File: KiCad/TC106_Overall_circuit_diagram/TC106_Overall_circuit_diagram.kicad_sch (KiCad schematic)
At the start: 52 parts, among them J1 JST_VH_01x05, J10 JST_VH_01x05, J1_24V1 JST_VH_01x04, J1_CN1 JST_VH_01x03, J2 JST_VH_01x05, J2_CN1 JST_VH_01x02, J3 JST_VH_01x05, J3_CN1 JST_VH_01x02, J4 JST_VH_01x05, J4_CN2 JST_VH_01x02, J5 JST_VH_01x05, J5_CN2 JST_VH_01x03, J6 JST_VH_01x05, J7 JST_VH_01x05, J8 JST_VH_01x05, J9 Conn_02x02_Odd_Even, Q1 DTC143E, Q2 DTC143E, Q3 2SD1863, Q5 DTC143E, U1 MC34063AP, U2 PIC16F73-ISP, U3 Dummy dsPic33FJ16MC102, U5 DC-DC_Converter

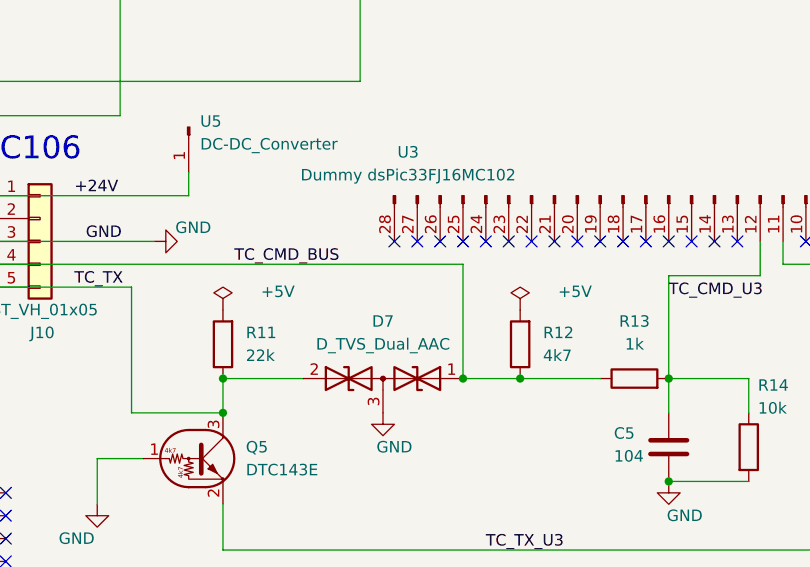
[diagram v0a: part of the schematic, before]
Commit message: UPDATE
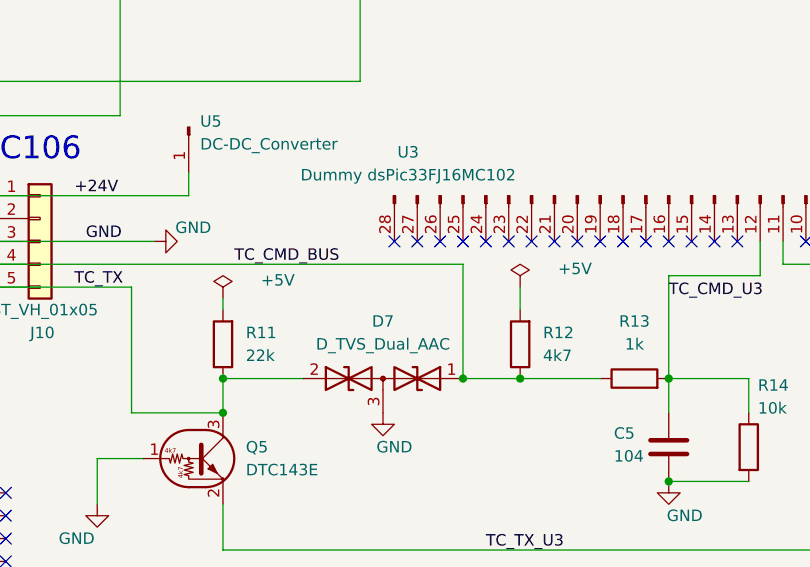
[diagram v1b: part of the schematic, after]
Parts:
- U3: footprint dsPIC33FJ16MC102:SOP65P780X200-28N -> dsPic33FJ16MC102:SOP65P780X200-28N
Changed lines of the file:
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@@
 	(wire
 		(pts
+			(xy 194.31 134.62) (xy 194.31 135.89)
+		)
+		(stroke
+			(width 0)
+			(type default)
+		)
+	)
+	(wire
+		(pts
 			(xy 129.54 142.24) (xy 151.13 142.24)
 		)
@@
 	(wire
 		(pts
+			(xy 227.33 133.35) (xy 227.33 135.89)
+		)
+		(stroke
+			(width 0)
+			(type default)
+		)
+	)
+	(wire
+		(pts
 			(xy 142.24 91.44) (xy 46.99 91.44)
 		)
@@
 	(symbol
 		(lib_id "power:PWR_FLAG")
-		(at 227.33 135.89 0)
+		(at 227.33 133.35 0)
 		(unit 1)
 		(exclude_from_sim no)
@@
 		(dnp no)
 		(property "Reference" "#U11_POWER_5V01"
-			(at 227.33 133.985 0)
+			(at 227.33 131.445 0)
 			(effects
 				(font
@@
 		)
 		(property "Value" "+5V"
-			(at 233.426 133.858 0)
+			(at 233.426 131.318 0)
 			(effects
 				(font
@@
 		)
 		(property "Footprint" ""
-			(at 227.33 135.89 0)
+			(at 227.33 133.35 0)
 			(effects
 				(font
@@
 		)
 		(property "Datasheet" "~"
-			(at 227.33 135.89 0)
+			(at 227.33 133.35 0)
 			(effects
 				(font
@@
 		)
 		(property "Description" "Special symbol for telling ERC where power comes from"
-			(at 227.33 135.89 0)
+			(at 227.33 133.35 0)
 			(effects
 				(font
@@
 			)
 		)
-		(property "Footprint" "dsPIC33FJ16MC102:SOP65P780X200-28N"
+		(property "Footprint" "dsPic33FJ16MC102:SOP65P780X200-28N"
 			(at 248.92 123.19 0)
 			(effects
@@
 	(symbol
 		(lib_id "power:PWR_FLAG")
-		(at 194.31 135.89 0)
+		(at 194.31 134.62 0)
 		(unit 1)
 		(exclude_from_sim no)
@@
 		(dnp no)
 		(property "Reference" "#U11_POWER_5V0101"
-			(at 194.31 133.985 0)
+			(at 194.31 132.715 0)
 			(effects
 				(font
@@
 		)
 		(property "Value" "+5V"
-			(at 200.406 133.858 0)
+			(at 200.406 132.588 0)
 			(effects
 				(font
@@
 		)
 		(property "Footprint" ""
-			(at 194.31 135.89 0)
+			(at 194.31 134.62 0)
 			(effects
 				(font
@@
 		)
 		(property "Datasheet" "~"
-			(at 194.31 135.89 0)
+			(at 194.31 134.62 0)
 			(effects
 				(font
@@
 		)
 		(property "Description" "Special symbol for telling ERC where power comes from"
-			(at 194.31 135.89 0)
+			(at 194.31 134.62 0)
 			(effects
 				(font
